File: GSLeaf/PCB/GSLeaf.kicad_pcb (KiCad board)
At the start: 2 copper layers, 46 x 103 mm, 129 parts, among them Q1 LED_5050, Q2 IRLML6401, Q3 IRLML9303, Q4 2N7002, SW1 SWITCH, SW2 BTN, SW3 BTN, SW4 BTN

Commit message: Tracing in progress
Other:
- net class Ant added: clearance 0.2, trace_width 0.3, via_dia 0.7, via_drill 0.3
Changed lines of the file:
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@@
     (links 394)
     (no_connects 393)
-    (area 111.961059 23.949999 158.032843 130.024011)
+    (area 111.961059 23.949999 158.032843 130.074011)
     (thickness 1.6)
     (drawings 55)
@@
     (uvia_dia 0.3)
     (uvia_drill 0.1)
-    (add_net +3.3V)
-    (add_net +5V)
-    (add_net +BATT)
     (add_net /ACC_INT1)
     (add_net /ACC_PWR)
@@
     (add_net /AU_SDIN)
     (add_net /AU_SDOUT)
-    (add_net /Antenna)
     (add_net /BAT_MEAS)
     (add_net /BLUE_LED)
@@
     (add_net /PN_RESET)
     (add_net /PN_SCK)
-    (add_net /PN_VDD)
-    (add_net /PWR_UNST_ALWAYS)
     (add_net /RED_LED)
     (add_net /RF1)
@@
     (add_net /SD_DAT2)
     (add_net /SD_DAT3)
-    (add_net /SD_PWR)
     (add_net /SD_PWR_EN)
     (add_net /SWCLK)
@@
     (add_net /UART_RX)
     (add_net /UART_TX)
-    (add_net GND)
     (add_net "Net-(C15-Pad1)")
     (add_net "Net-(C16-Pad1)")
@@
     (add_net "Net-(XL2-PadH3)")
     (add_net "Net-(XL2-PadH4)")
-    (add_net PwrMCU)
-    (add_net PwrUnst)
-    (add_net VAA)
-    (add_net VCC)
+  )
+  (net_class Ant ""
+    (clearance 0.2)
+    (trace_width 0.3)
+    (via_dia 0.7)
+    (via_drill 0.3)
+    (uvia_dia 0.3)
+    (uvia_drill 0.1)
+    (add_net /Antenna)
   )
   (net_class Wide ""
@@
     (uvia_dia 0.3)
     (uvia_drill 0.1)
+    (add_net +3.3V)
+    (add_net +5V)
+    (add_net +BATT)
+    (add_net /PN_VDD)
+    (add_net /PWR_UNST_ALWAYS)
+    (add_net /SD_PWR)
+    (add_net GND)
+    (add_net PwrMCU)
+    (add_net PwrUnst)
+    (add_net VAA)
+    (add_net VCC)
   )
   (module Installation:BATTERY_AAA_X3 (layer F.Cu)

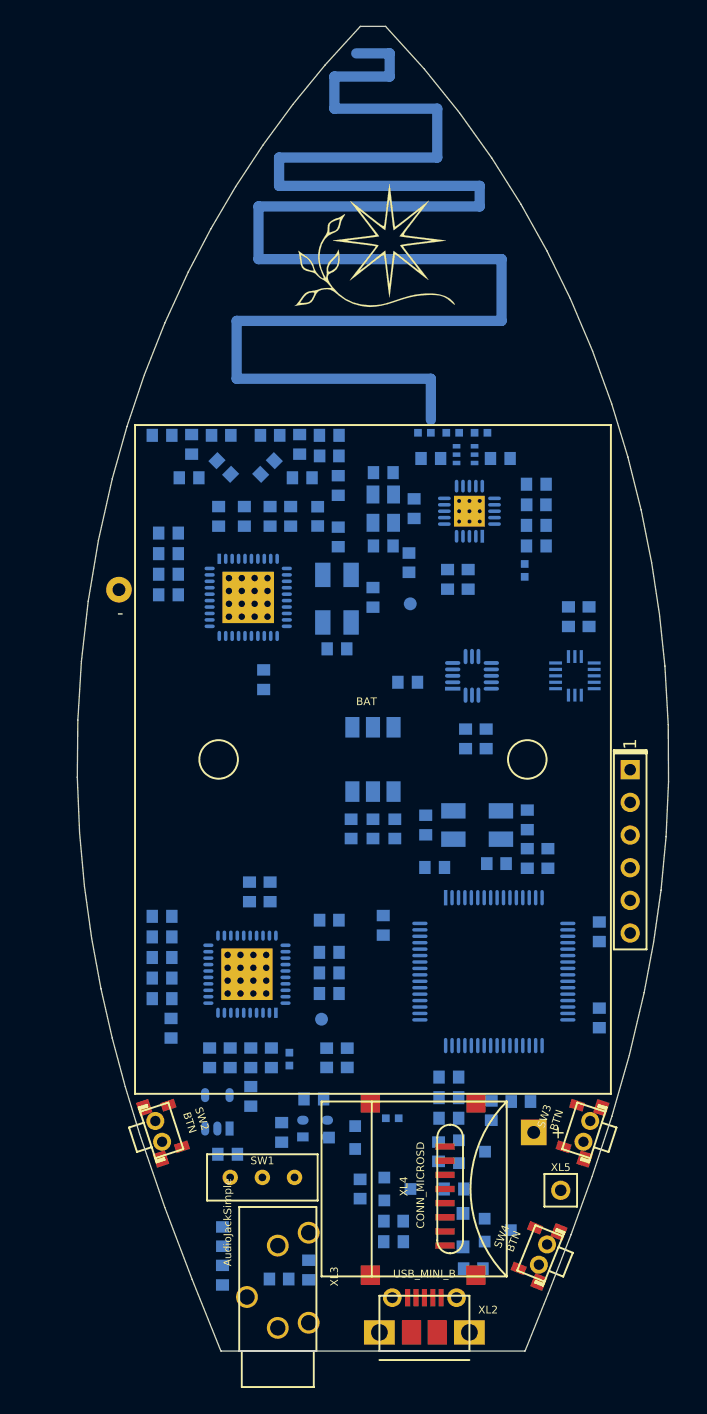
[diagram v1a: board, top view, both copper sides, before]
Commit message: Sent to factory
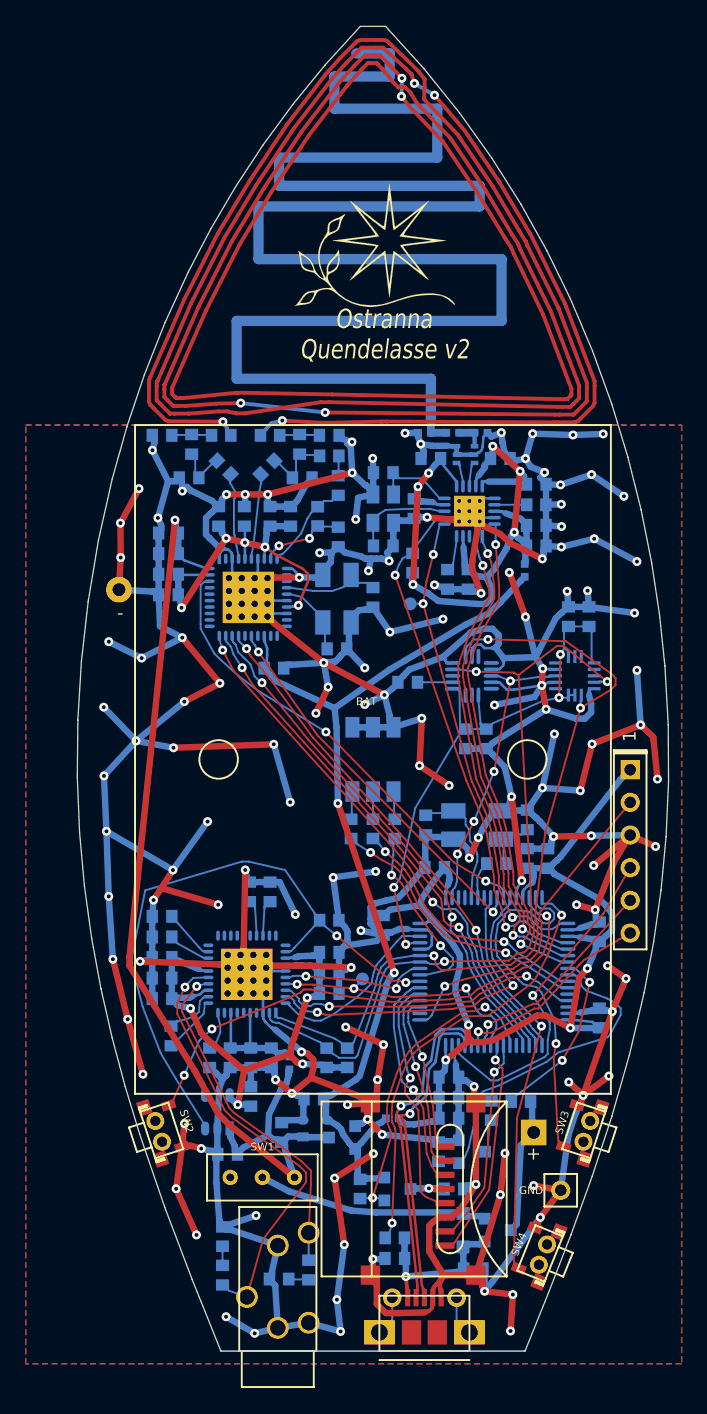
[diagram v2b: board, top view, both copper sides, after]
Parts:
- moved TP1 4.47 mm to (134.2, 98.1)
- moved C1 1.30 mm to (136.7, 119.8)
- moved R11 1.30 mm to (136.7, 118.2)
- moved C54 1.20 mm to (127.3, 73.9), turned to 0 degrees
- moved C16 0.60 mm to (119.3, 102.5)
- moved L2 0.30 mm to (128.5, 104.6)
- moved R13 0.28 mm to (138.1, 65.7)
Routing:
- net GND: track 0.00 -> 758.8 mm, vias 0 -> 138
- net /Antenna: track 0.00 -> 393.1 mm, vias 0 -> 8
- net /ANT2: track 0.00 -> 141.3 mm
- net PwrMCU: track 0.00 -> 89.5 mm, vias 0 -> 6
- net PwrUnst: track 0.00 -> 80.2 mm, vias 0 -> 1
- net +3.3V: track 0.00 -> 73.1 mm, vias 0 -> 2
- net /SDA: track 0.00 -> 64.3 mm, vias 0 -> 3
- net /SCL: track 0.00 -> 63.3 mm, vias 0 -> 3
- net VCC: track 0.00 -> 61.2 mm, vias 0 -> 6
- net /AU_RST: track 0.00 -> 49.3 mm, vias 0 -> 2
- net VAA: track 0.00 -> 48.2 mm, vias 0 -> 4
- net /PN_SCK: track 0.00 -> 41.3 mm, vias 0 -> 2
- net /PN_MISO: track 0.00 -> 40.5 mm, vias 0 -> 2
- net /CC_CS: track 0.00 -> 40.5 mm, vias 0 -> 2
- net /PN_NSS: track 0.00 -> 40.1 mm, vias 0 -> 2
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- added copper zone on B.Cu, net GND
- added copper zone on F.Cu, net GND
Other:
- board text added: "Audio"
- board text added: "GND"
- board text added: "NFC"
- board text added: "Ostranna"
- board text added: "Quendelasse v2"
- board text added: "Radio"
